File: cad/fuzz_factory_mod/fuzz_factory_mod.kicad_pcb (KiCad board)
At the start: 2 copper layers, 138 x 114 mm, 390 parts, among them J101 Conn_interface_1, J102 Conn_interface_2, J1701 Barrel_Jack_Switch, J1702 Conn_Battery, J1703 CONN_AUDIO_IN, J1704 CONN_AUDIO_OUT, J201 Conn_MCU_SWD, J2801 CONN_AUDIO_OUT_REF, J2802 CONN_EXP_1, J2803 CONN_EXP_2, J301 USB_B_Micro, J401 USB_B_Micro, J901 CONN_MIDI_IN, J902 CONN_MIDI_THRU, J903 CONN_MIDI_OUT, J904 Conn_01x10_Female, J905 Conn_01x10_Female, K2101 Fujitsu-Takamisawa-A_AL, Q1301 MMDT3904, Q1302 MMDT3904, Q1602 DTA123Y, Q1603 DTA123Y, Q1604 DTA123Y, Q1605 DTA123Y, Q1701 DTC114Y, Q1702 DTA114E, Q2201 BCP51, Q601 DTA123Y, Q602 DTA123Y, Q603 DTA123Y, Q604 DTA123Y, Q801 MMDT3904, Q802 MMDT3904, SW1101 SW_PUSH, SW1201 SW_PUSH, SW1301 SW_PUSH, U1101 LM1458, U1102 MC33202, U1201 LM2903, U1202 MC33202, U1501 LM1458, U1502 MC33202, U1503 MC33202, U1601 4050, U1602 4049, U1603 4504, U1604 MC33202, U1701 LM1458, U1702 MC33202, U1803 LM1458, U1804 MC33202, U1901 LM2903, U201 STM32F303VCTx, U2201 TL072, U2202 LM2674M-ADJ, U2203 LM78L05_SO8, U301 USBLC6-2SC6, U302 FT230XS, U401 USBLC6-2SC6, U501 74LS132, U601 4050, U602 4504, U603 MC33202, U604 4049, U701 AD5262_ABC, U901 4N25, Y201 Resonator_Small

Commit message: Continued layout.
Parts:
- moved C2211 304.2 mm to (234.6, 109.4), turned to 0 degrees
- moved C2202 284.5 mm to (225.7, 109.4)
- moved C2206 277.4 mm to (225.7, 116.0), turned to 0 degrees
- moved R1702 273.0 mm to (102.2, 49.8)
- moved C210 270.5 mm to (139.8, 90.8), turned to 0 degrees
- moved R207 267.4 mm to (136.8, 90.8), turned to 0 degrees
- moved R1505 262.2 mm to (97.8, 106.2), turned to 270 degrees
- moved D1701 257.7 mm to (79.8, 42.0)
- moved R808 254.7 mm to (104.8, 64.2), turned to 0 degrees
- moved Q1701 254.5 mm to (80.8, 46.8), turned to 180 degrees
- moved R815 254.4 mm to (104.8, 65.9), turned to 0 degrees
- moved R807 254.2 mm to (104.8, 67.7), turned to 0 degrees
- moved K2101 253.6 mm to (69.5, 46.8), turned to 0 degrees
- moved R1510 253.4 mm to (92.2, 125.5), turned to 90 degrees
- moved R1306 253.4 mm to (129.5, 104.5), turned to 0 degrees
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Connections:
- C907 pad 2: +5V -> /MCU/MIDI/+5V_IN
- R205 pad 1: +5V -> /MCU/MIDI/+5V_IN
- R206 pad 1: +5V -> /MCU/MIDI/+5V_IN
- R918 pad 2: +5V -> /MCU/MIDI/+5V_IN
- R920 pad 1: +5V -> /MCU/MIDI/+5V_IN
- R922 pad 1: +5V -> /MCU/MIDI/+5V_IN
- U501 pad 14: +5V -> /MCU/MIDI/+5V_IN
- U901 pad 6: +5V -> /MCU/MIDI/+5V_IN
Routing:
- net +3V3: track 88.2 -> 4.71 mm, vias 2 -> 0
- net BYPASS_CMD: track 0.00 -> 82.0 mm, vias 0 -> 4
- net DISP_ENABLE: track 0.00 -> 80.5 mm, vias 0 -> 2
- net SPI2_MOSI: track 0.00 -> 77.3 mm, vias 0 -> 2
- net SPI2_SCK: track 0.00 -> 76.5 mm, vias 0 -> 2
- net /CONNECTORS/AUDIO_IN_CONN: track 0.00 -> 67.2 mm
- net GNDD: track 16.9 -> 59.5 mm, vias 5 -> 16
- net ENC3_IN_CW: track 0.00 -> 34.8 mm
- net ENC3_IN_CCW: track 0.00 -> 34.7 mm
- net ENC1_IN_CCW: track 0.00 -> 34.6 mm, vias 0 -> 2
- net /CONNECTORS/AUDIO_OUT_CONN: track 0.00 -> 34.0 mm
- net DISP_LATCH: track 0.00 -> 33.3 mm, vias 0 -> 2
- net +9V: track 22.9 -> 54.0 mm
- net ENC1__LED_GREEN: track 0.00 -> 30.0 mm, vias 0 -> 2
- net ENC1_IN_CW: track 0.00 -> 28.7 mm, vias 0 -> 2
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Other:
- board text added: "0.5mm clearance with enclosure wall"

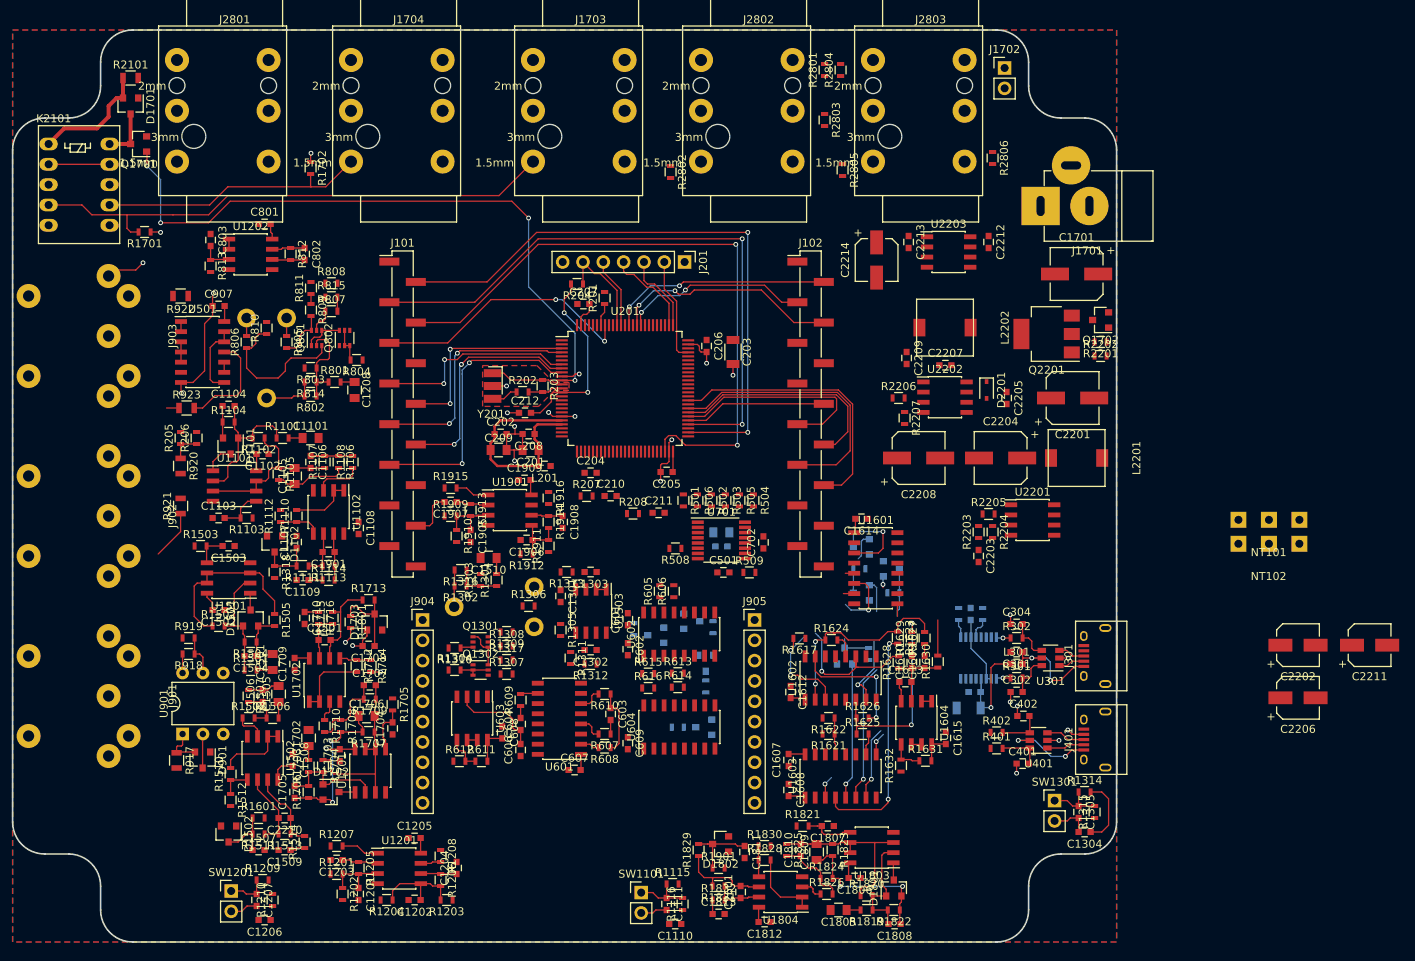
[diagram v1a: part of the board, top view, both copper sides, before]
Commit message: Continued layout.
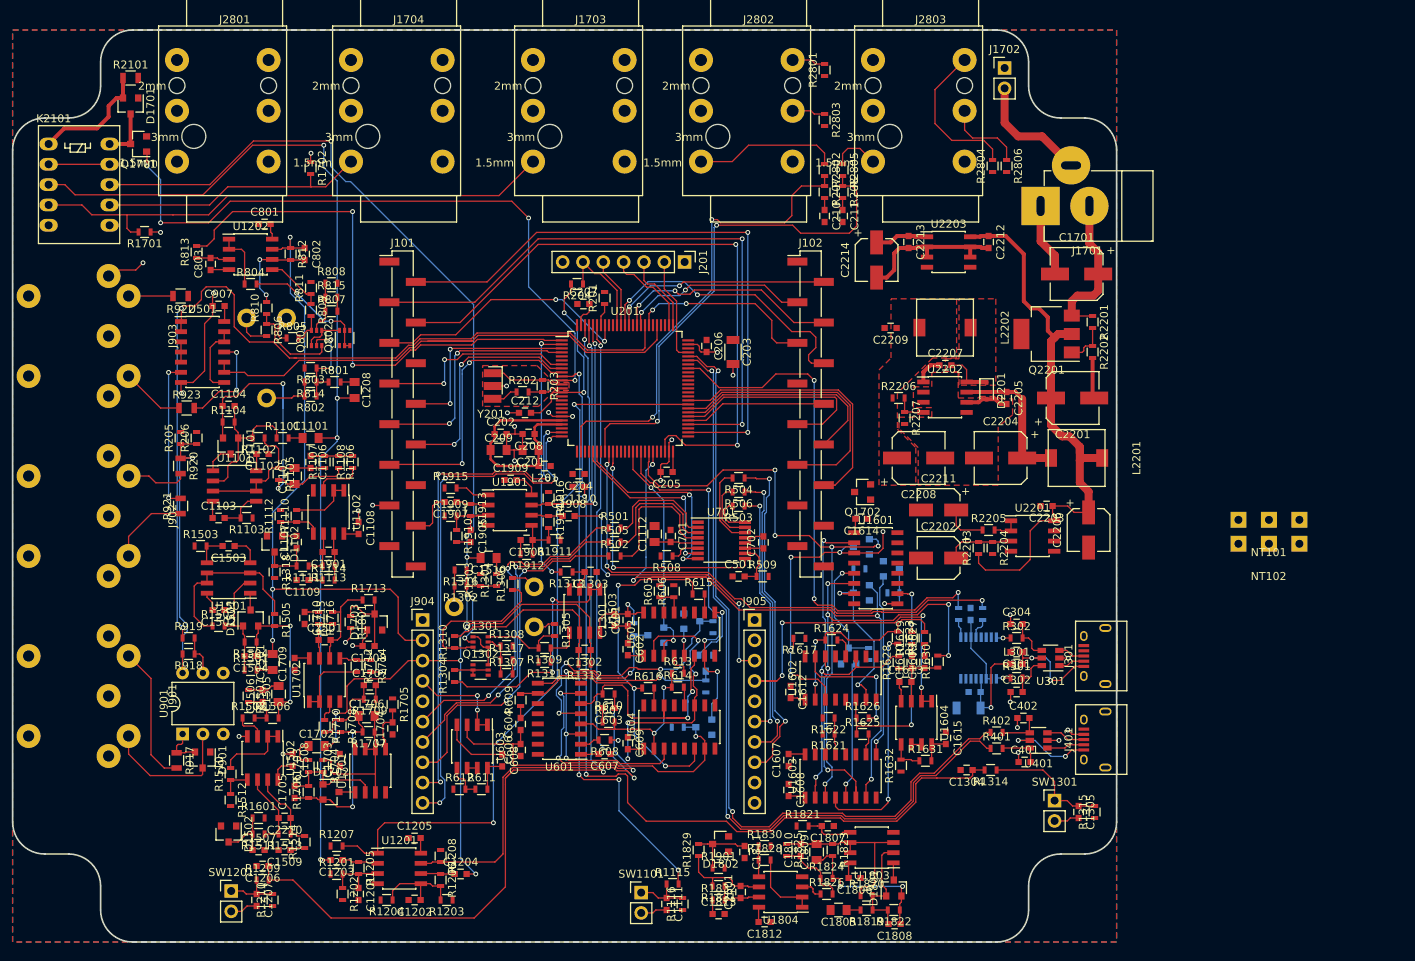
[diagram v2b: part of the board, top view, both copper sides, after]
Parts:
- C1112, C701: moved to F.Cu
- moved C2211 56.5 mm to (180.8, 92.5), turned to 180 degrees
- moved C1110 56.0 mm to (135.8, 89.6)
- moved R207 48.3 mm to (166.5, 52.8), turned to 270 degrees
- moved R208 48.0 mm to (168.8, 52.8), turned to 270 degrees
- moved C2202 46.2 mm to (180.8, 98.5), turned to 180 degrees
- moved C210 44.1 mm to (166.5, 55.8), turned to 270 degrees
- moved C211 43.7 mm to (168.8, 55.8), turned to 270 degrees
- moved Q1702 36.7 mm to (171.2, 90.2)
- moved C2206 33.5 mm to (199.5, 95.0), turned to 270 degrees
- moved R2804 22.5 mm to (187.5, 49.5)
- moved R2802 19.3 mm to (166.5, 50.0)
- moved C1304 16.7 mm to (184.2, 125.0)
- moved R505 16.4 mm to (140.2, 96.5), turned to 0 degrees
- moved R804 16.3 mm to (94.8, 64.2), turned to 0 degrees
- moved R502 14.0 mm to (140.2, 98.2), turned to 0 degrees
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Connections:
- net Net-(C2207-Pad2) renamed /PSU/DCDC_VSW
- J102 pad 5: ENC2_IN_CCW -> ENC2_IN_CW
- U201 pad 82: ENC2_IN_CCW -> ENC2_IN_CW
- U201 pad 92: ENC2_IN_CCW -> (no net)
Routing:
- net AUDIO_OUT_FX: track 0.00 -> 182.0 mm, vias 0 -> 7
- net AUDIO_IN_FX: track 0.00 -> 134.1 mm, vias 0 -> 4
- net /MCU/SW_PRESET_UP: track 0.00 -> 119.3 mm, vias 0 -> 2
- net /MCU/UART5_RX: track 1.27 -> 115.8 mm, vias 0 -> 2
- net /MCU/SW_PRESET_DOWN: track 8.50 -> 116.8 mm, vias 0 -> 2
- net USB_DP: track 0.00 -> 100.6 mm, vias 0 -> 2
- net USB_DM: track 0.00 -> 100.1 mm, vias 0 -> 2
- net INPUT_CAPTURE_2: track 2.54 -> 96.7 mm, vias 0 -> 2
- net INPUT_CAPTURE_1: track 4.76 -> 93.8 mm, vias 0 -> 2
- net /ANALOG/IN_AUDIO_VCA: track 4.12 -> 84.0 mm, vias 0 -> 3
- net Net-(C2201-Pad1): track 0.00 -> 75.4 mm
- net /MCU/SW_BYPASS: track 2.30 -> 76.0 mm, vias 1 -> 5
- net Ref_Stab_DAC_PWM_MSB: track 13.2 -> 84.6 mm, vias 1 -> 4
- net Ref_Stab_DAC_PWM_LSB: track 6.32 -> 76.0 mm, vias 1 -> 5
- net VCA_IN_PWM: track 0.00 -> 68.7 mm, vias 0 -> 2
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- added copper zone on F.Cu, net +3V3
- added copper zone on F.Cu, net /PSU/DCDC_VSW
